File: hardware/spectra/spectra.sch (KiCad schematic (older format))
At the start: 21 parts, among them J1 Output, J2 Ext Coil, J3 Ext Shunt, J4 Coil, J5 Mix Shunt, U1 TLV170DBV

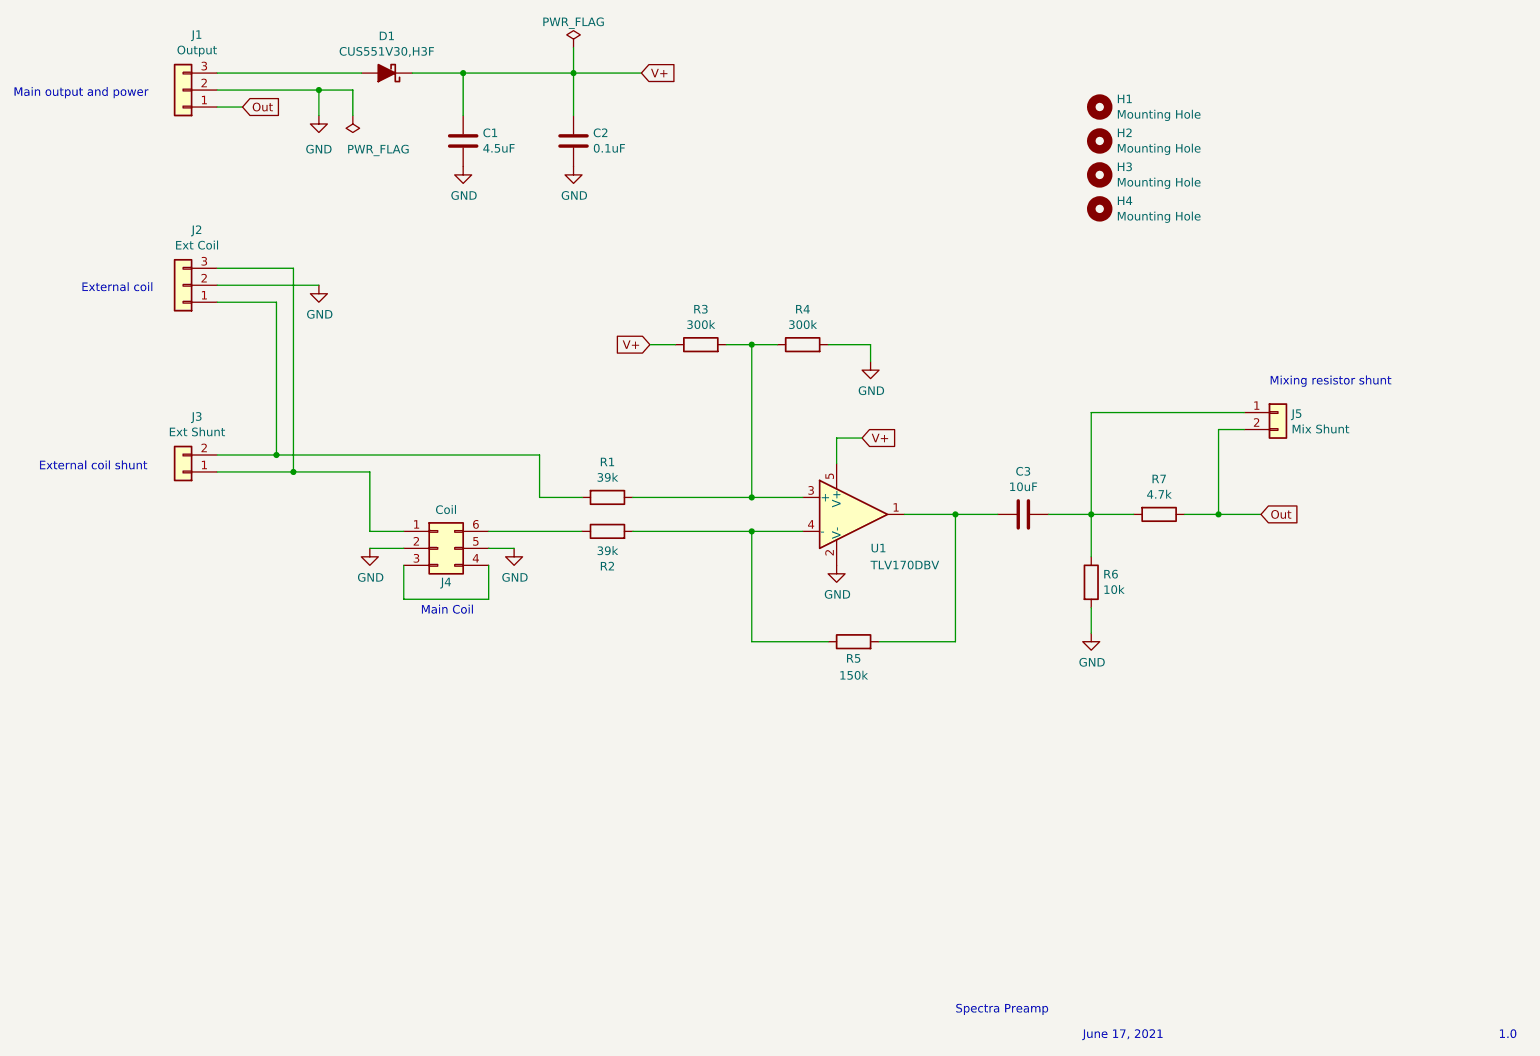
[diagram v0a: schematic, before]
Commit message: Fully routed
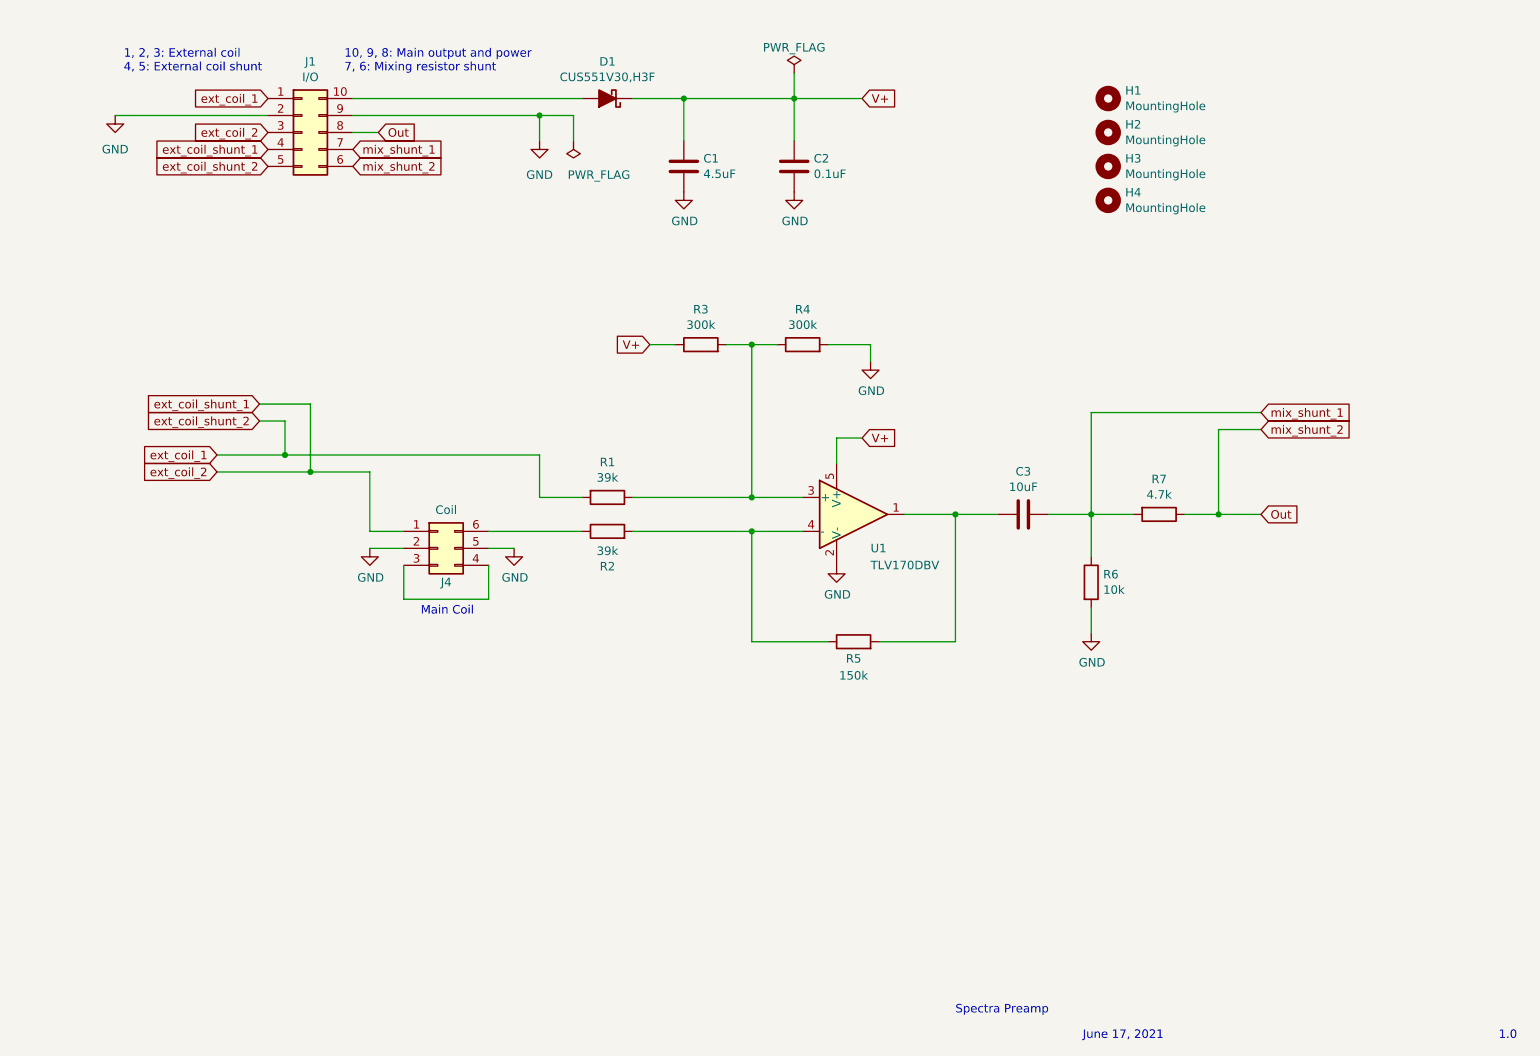
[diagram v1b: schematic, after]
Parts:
- removed J1: Output, Connector_Harwin:Harwin_M20-89003xx_1x03_P2.54mm_Horizontal, symbol Connector_Generic:Conn_01x03
- removed J2: Ext Coil, Connector_Harwin:Harwin_M20-89003xx_1x03_P2.54mm_Horizontal, symbol Connector_Generic:Conn_01x03
- removed J3: Ext Shunt, Connector_PinSocket_2.00mm:PinSocket_1x02_P2.00mm_Vertical, symbol Connector_Generic:Conn_01x02
- removed J5: Mix Shunt, Connector_PinSocket_2.00mm:PinSocket_1x02_P2.00mm_Vertical, symbol Connector_Generic:Conn_01x02
- added J1: I/O, cycfi_library:pin_header_2x5p_2.54mm_smd_horizontal, symbol Connector_Generic:Conn_02x05_Counter_Clockwise
- H1, H2, H3, H4: value Mounting Hole -> MountingHole; footprint MountingHole:MountingHole_2mm -> cycfi_library:mounting_hole_2.1mm
- J4: footprint Connector_PinSocket_1.00mm:PinSocket_2x03_P1.00mm_Vertical_SMD -> cycfi_library:pin_socket_2x3p_1.00mm_smd_vertical
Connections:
- net GND: now also J1.2 (Pin_2), J1.9 (Pin_9)
- net Out: now also J1.6 (Pin_6), J1.8 (Pin_8)
- net ext_coil_2: now reaches J4.1 (Pin_1)
- net ext_coil_2: now also J1.3 (Pin_3), J1.4 (Pin_4)
- net ext_coil_1: now reaches R1.2
- net ext_coil_1: now also J1.1 (Pin_1), J1.5 (Pin_5)
- net at D1.2 (A): now also J1.10 (Pin_10)
- net mix_shunt_1: now reaches C3.1, R6.1, R7.2
- net mix_shunt_1: now also J1.7 (Pin_7)
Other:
- note added: "1, 2, 3: External coil\n4, 5: External coil shunt"
- note added: "10, 9, 8: Main output and power\n7, 6: Mixing resistor shunt"
- note removed: "External coil"
- note removed: "External coil shunt"
- note removed: "Main output and power"
- note removed: "Mixing resistor shunt"
- moved on the sheet: C1, C2, D1

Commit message: Merge branch 'reversed' into master
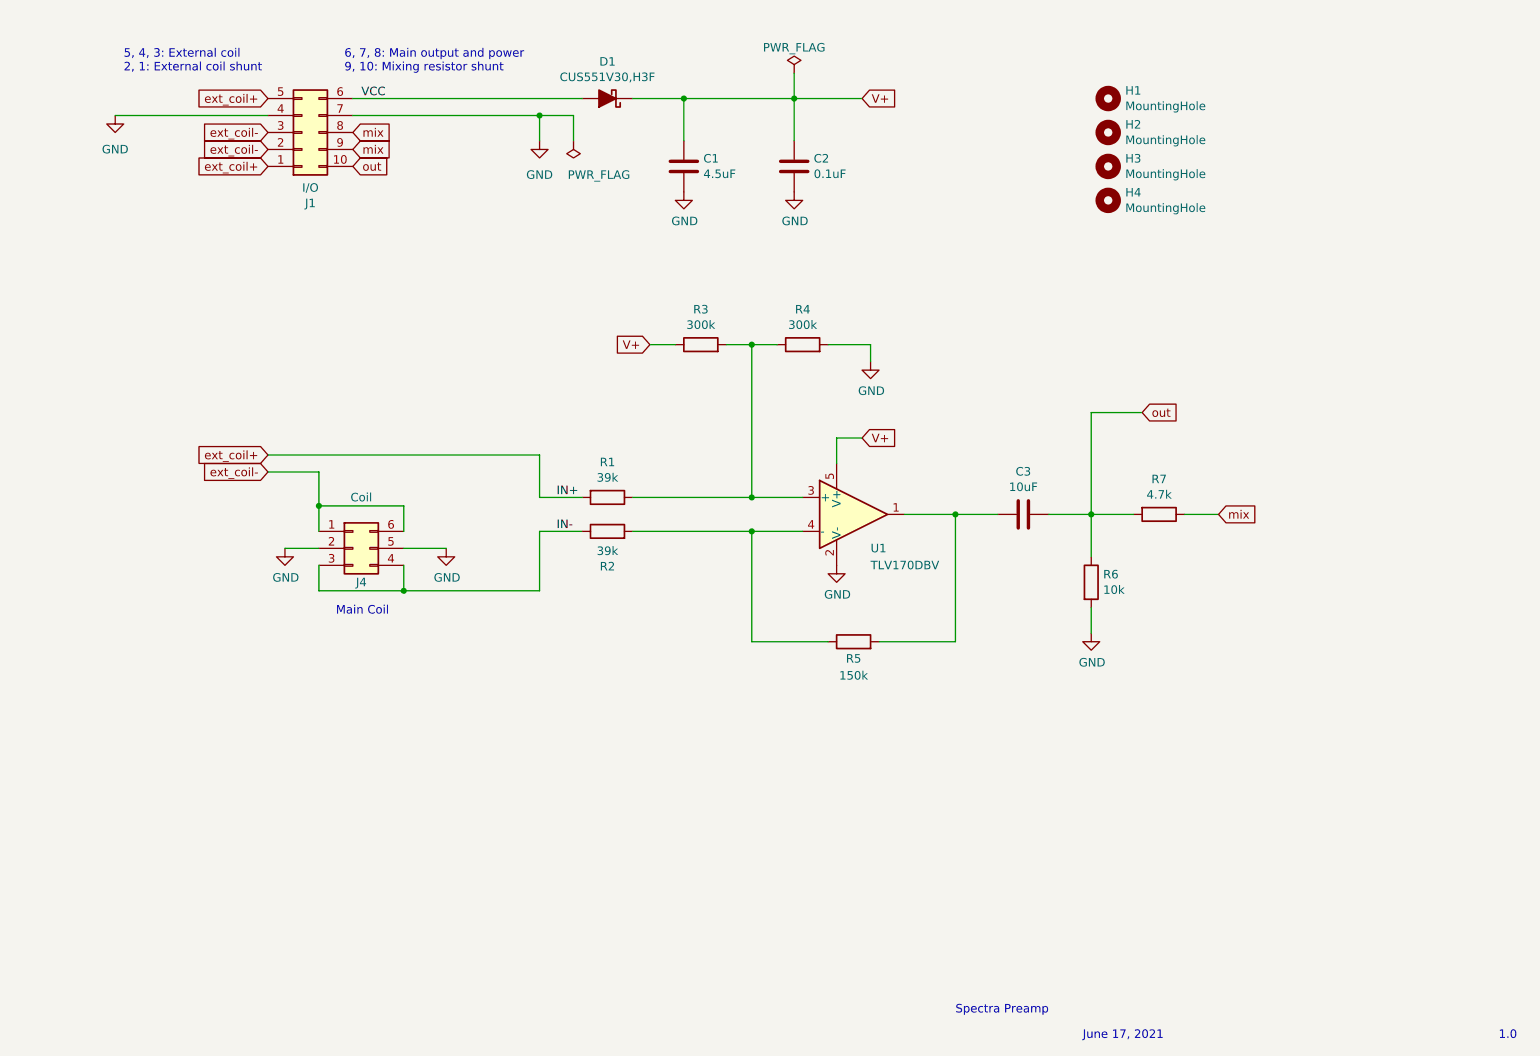
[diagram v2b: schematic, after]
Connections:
- net GND: now also J1.4 (Pin_4), J1.7 (Pin_7); no longer J1.2 (Pin_2), J1.9 (Pin_9)
- net IN-: now reaches J4.3 (Pin_3), J4.4 (Pin_4)
- net IN-: now also R2.1
- net ext_coil-: now reaches J4.6 (Pin_6)
- net ext_coil-: now also J1.2 (Pin_2), J1.3 (Pin_3), J4.1 (Pin_1); no longer R2.1
- net VCC: now reaches D1.2 (A)
- net VCC: now also J1.6 (Pin_6); no longer J1.10 (Pin_10)
- net Out renamed mix
- net mix: now also J1.9 (Pin_9); no longer J1.6 (Pin_6)
- net ext_coil_1 renamed ext_coil+
- removed net ext_coil_2: J1.3 (Pin_3), J1.4 (Pin_4), J4.1 (Pin_1)
- net mix_shunt_1 renamed out
- net out: now also J1.10 (Pin_10); no longer J1.7 (Pin_7)
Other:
- note added: "5, 4, 3: External coil\n2, 1: External coil shunt"
- note added: "6, 7, 8: Main output and power\n9, 10: Mixing resistor shunt"
- note removed: "1, 2, 3: External coil\n4, 5: External coil shunt"
- note removed: "10, 9, 8: Main output and power\n7, 6: Mixing resistor shunt"
- moved on the sheet: J4
